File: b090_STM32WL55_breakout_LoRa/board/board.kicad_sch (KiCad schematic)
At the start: 14 parts, among them J1 DebugEdge_02x05, J2 SPI_2x3, J4 UART_2x2, J7 I2C_2x2, J8 UART_2x2, J9 ADC_2x3

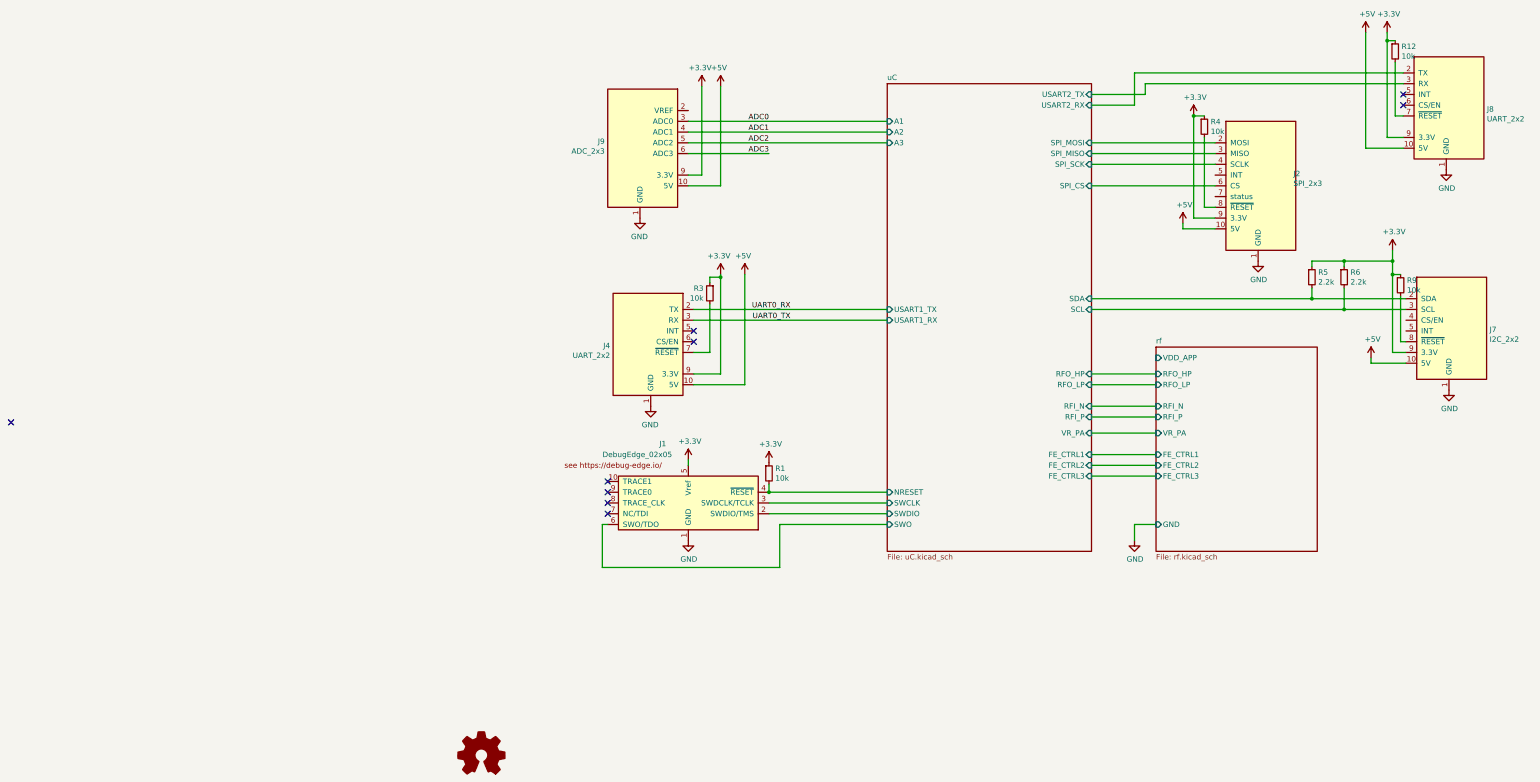
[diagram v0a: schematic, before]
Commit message: dev board cloned
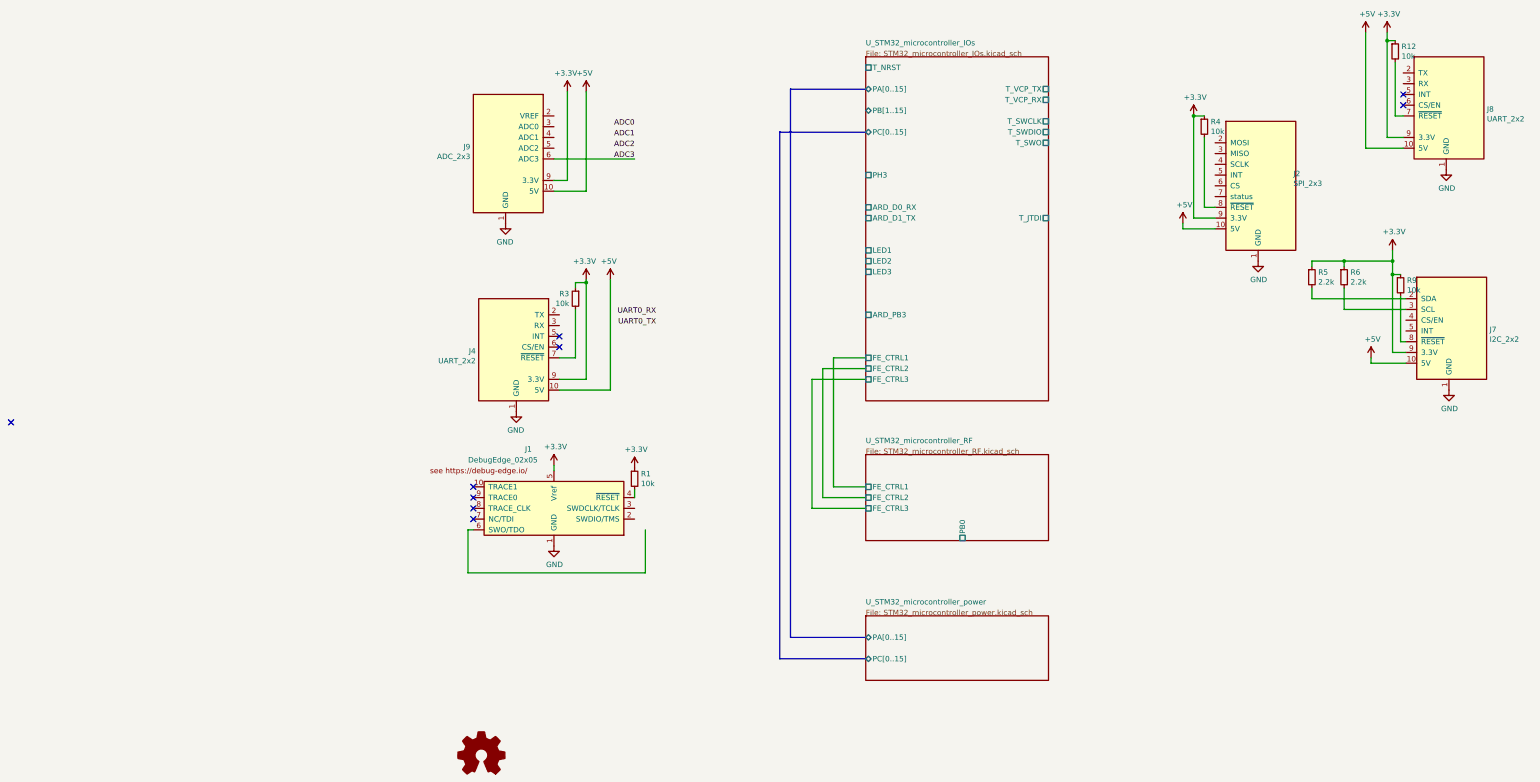
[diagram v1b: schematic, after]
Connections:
- net ADC0: no longer J9.3 (ADC0)
- net ADC1: no longer J9.4 (ADC1)
- net ADC2: no longer J9.5 (ADC2)
- net UART0_RX: no longer J4.2 (TX)
- net UART0_TX: no longer J4.3 (RX)
- net uC/NRESET: no longer names the net of J1.4 (~{RESET}), R1.2
- net uC/SCL: no longer names the net of J7.3 (SCL), R6.2
- net uC/SDA: no longer names the net of J7.2 (SDA), R5.2
- net uC/SPI_CS: no longer names the net of J2.6 (CS)
- net uC/SPI_MISO: no longer names the net of J2.3 (MISO)
- net uC/SPI_MOSI: no longer names the net of J2.2 (MOSI)
- net uC/SPI_SCK: no longer names the net of J2.4 (SCLK)
- net uC/SWCLK: no longer names the net of J1.3 (SWDCLK/TCLK)
- net uC/SWDIO: no longer names the net of J1.2 (SWDIO/TMS)
- net uC/SWO: no longer names the net of J1.6 (SWO/TDO)
- net uC/USART2_RX: no longer names the net of J8.2 (TX)
- net uC/USART2_TX: no longer names the net of J8.3 (RX)
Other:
- removed sheet rf
- removed sheet uC
- added sheet U_STM32_microcontroller_IOs (STM32_microcontroller_IOs.kicad_sch)
- added sheet U_STM32_microcontroller_RF (STM32_microcontroller_RF.kicad_sch)
- added sheet U_STM32_microcontroller_power (STM32_microcontroller_power.kicad_sch)
- moved on the sheet: J1, J4, J9, R1, R3
